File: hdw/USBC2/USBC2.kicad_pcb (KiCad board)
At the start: 2 copper layers, 14 x 17.8 mm, 10 parts, among them J1 Conn_01x02, J3 Conn_01x02, J6 Conn_01x02, P1 USB_C_2.0

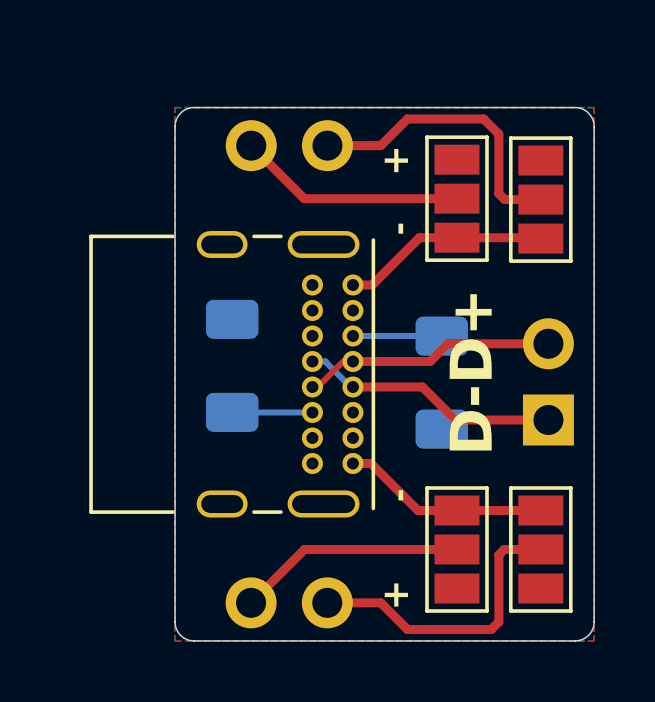
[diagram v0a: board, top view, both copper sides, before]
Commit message: Save changes at: 1748460734
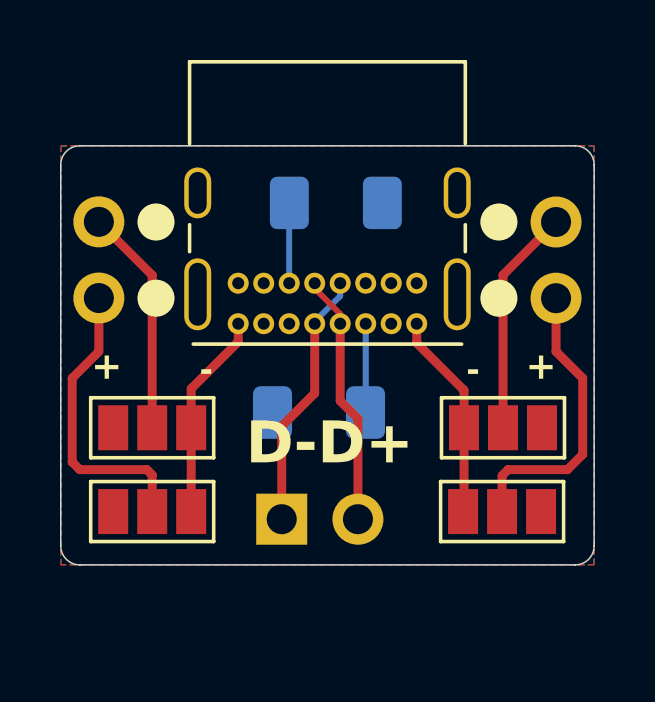
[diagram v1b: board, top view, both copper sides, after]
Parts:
- moved J6 13.7 mm to (81.3, 114.3), turned to 180 degrees
- moved JP8 13.0 mm to (83.1, 124.0), turned to 180 degrees
- moved JP7 10.9 mm to (83.1, 121.2), turned to 180 degrees
- moved JP6 10.5 mm to (94.7, 124.0), turned to 0 degrees
- moved J1 10.5 mm to (96.5, 114.3), turned to 180 degrees
- moved J3 9.49 mm to (87.4, 124.2), turned to -90 degrees
- moved JP5 7.79 mm to (94.8, 121.2), turned to 0 degrees
- moved R2 6.44 mm to (89.2, 113.7), turned to 0 degrees
- moved R1 4.21 mm to (88.6, 120.7), turned to 180 degrees
- moved P1 2.49 mm to (91.9, 117.7), turned to 180 degrees
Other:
- board size 14 x 17.8 mm -> 17.8 x 14 mm

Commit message: Save changes at: 1751310596
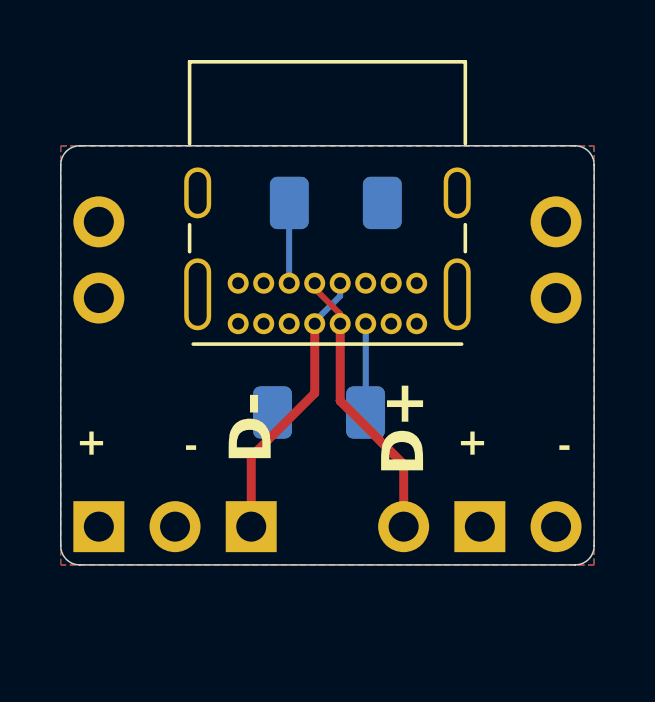
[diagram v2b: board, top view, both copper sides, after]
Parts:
- removed JP5, JP6, JP7, JP8: SolderJumper_3_Open, Jumper:SolderJumper-3_P1.3mm_Open_Pad1.0x1.5mm
- added J2: Conn_01x02, Connector_PinHeader_2.54mm:PinHeader_1x02_P2.54mm_Vertical, B.Cu at (81.3, 116.8)
- added J4: Conn_01x02, Connector_PinHeader_2.54mm:PinHeader_1x02_P2.54mm_Vertical, B.Cu at (96.5, 114.3)
- moved J1 10.5 mm to (94.0, 124.5), turned to -90 degrees
- moved J6 10.2 mm to (81.3, 124.5), turned to -90 degrees
- moved J3 1.05 mm to (86.4, 124.5)
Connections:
- J1 pad 1: Net-(J1-Pin_1) -> VCC
- J1 pad 2: Net-(J1-Pin_2) -> GND
- J6 pad 1: Net-(J6-Pin_1) -> VCC
- J6 pad 2: Net-(J6-Pin_2) -> GND
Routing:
- net GND: track 13.8 -> 0.00 mm
- net Net-(J6-Pin_2): track 9.90 -> 0.00 mm
- net Net-(J1-Pin_2): track 9.75 -> 0.00 mm
- net Net-(J6-Pin_1): track 7.60 -> 0.00 mm
- net Net-(J1-Pin_1): track 7.59 -> 0.00 mm
- net D+: track 8.46 -> 9.10 mm
